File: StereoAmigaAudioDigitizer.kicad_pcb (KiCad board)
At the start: 2 copper layers, 54.4 x 44.7 mm, 22 parts, among them J1 RIGHT, J2 LEFT, J3 DB25_Male, U1 MCP6002, U2 DG419LDJ, U3 ADC0820CCN+

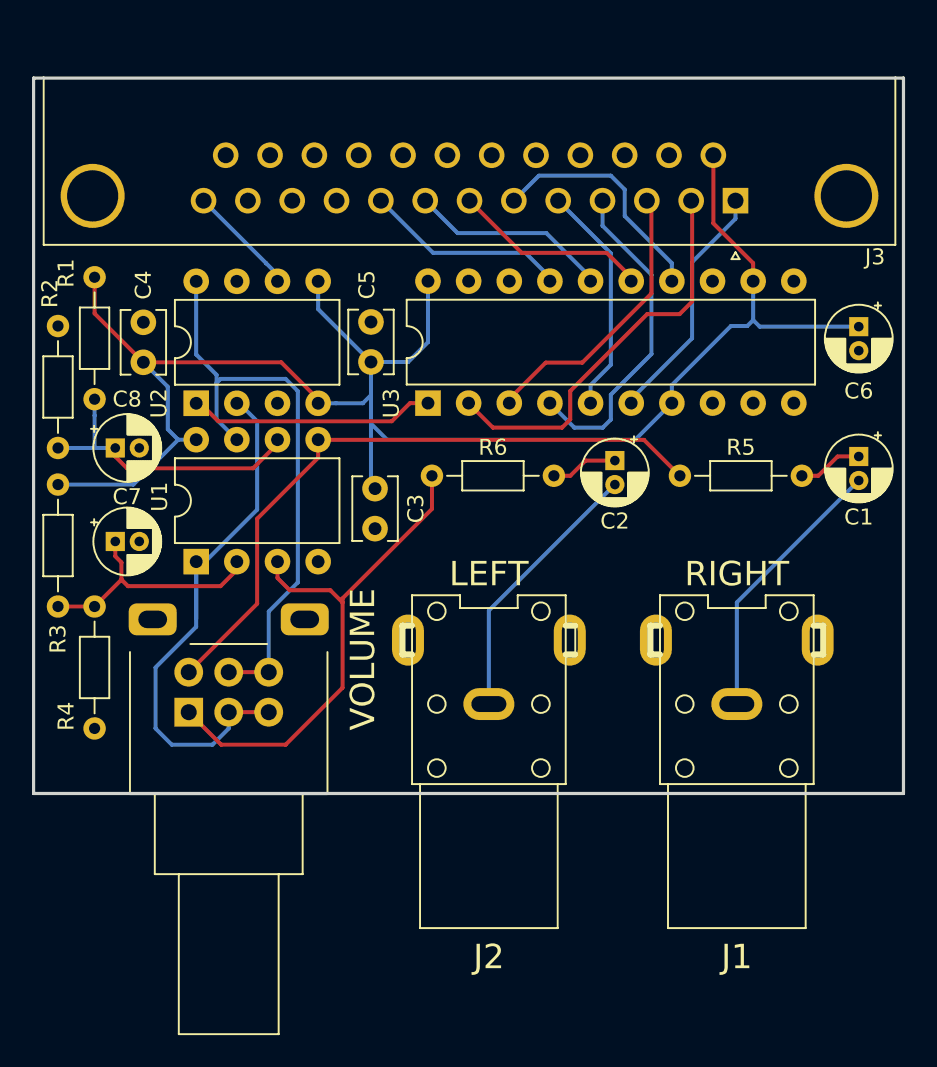
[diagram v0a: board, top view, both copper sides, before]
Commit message: Add files via upload
Modified PCB
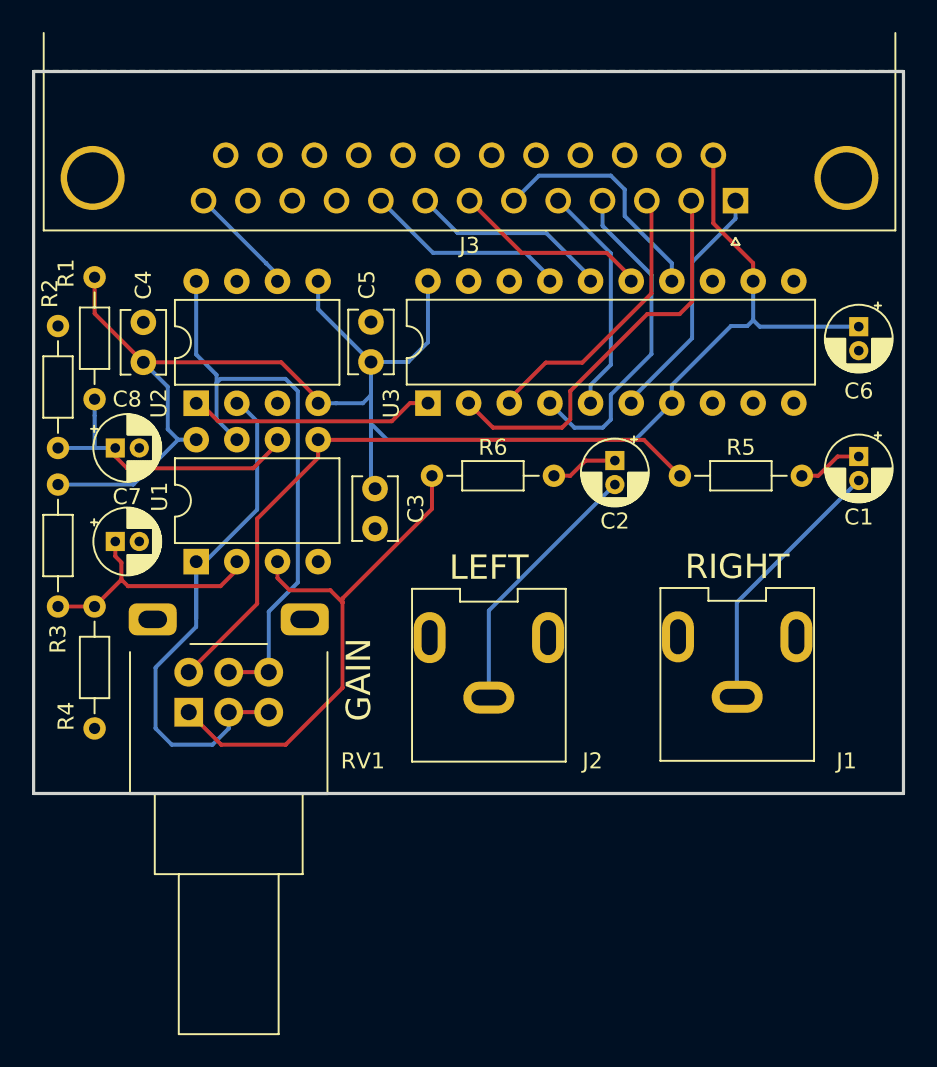
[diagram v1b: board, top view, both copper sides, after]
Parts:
- J1: footprint w_conn_av:rca_red -> w_conn_av:rca_white
- J3: footprint Connector_Dsub:DSUB-25_Male_Horizontal_P2.77x2.84mm_EdgePinOffset4.94mm_Housed_MountingHolesOffset7.48mm -> Connector_Dsub:DSUB-25_Male_Horizontal_P2.77x2.84mm_EdgePinOffset7.70mm_Housed_MountingHolesOffset9.12mm
- moved J1 0.45 mm to (140.5, 86.2)
- moved J2 0.40 mm to (125.0, 86.2)
- renumbered VOLUME to RV1
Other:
- board size 54.4 x 44.7 mm -> 54.4 x 45.1 mm
- board text added: "AMIGA STEREO DIGITIZER V1.2"
- board text added: "GAIN"
- board text removed: "AMIGA STEREO DIGITIZER V1.1"
